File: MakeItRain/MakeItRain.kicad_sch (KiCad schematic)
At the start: 13 parts, among them IC1 DS3231SN#, J1 Conn_02x16_Odd_Even, J2 Conn_02x19_Odd_Even, J3 Conn_01x19, U2 S8411-45R

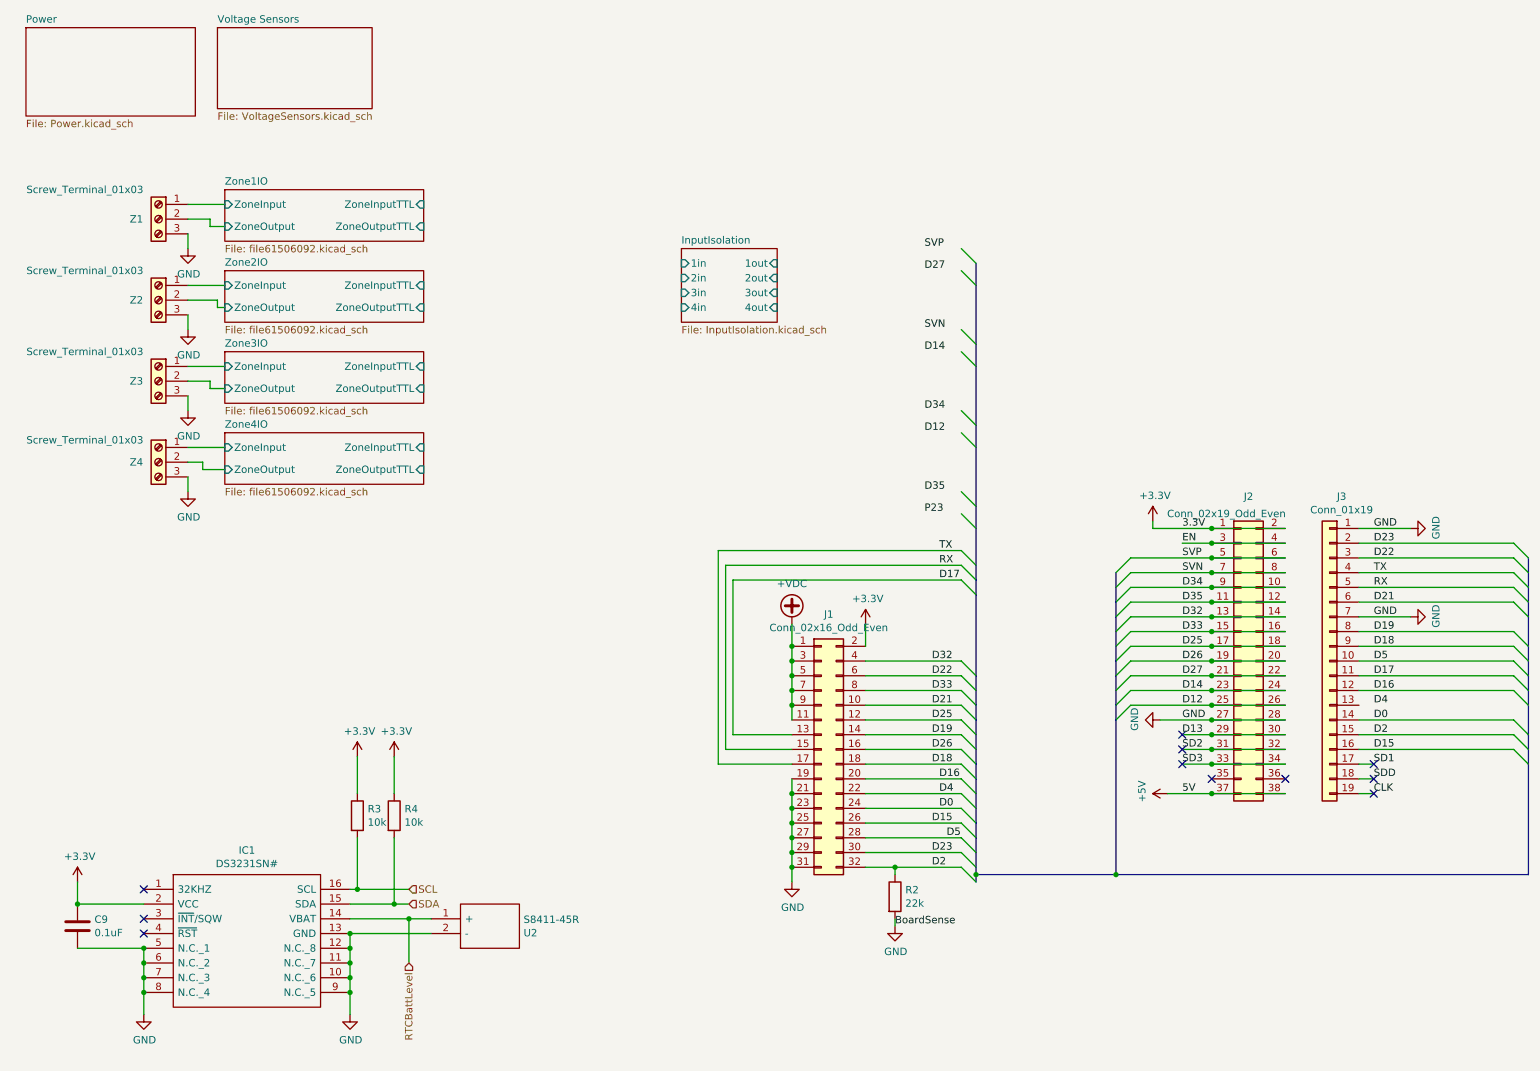
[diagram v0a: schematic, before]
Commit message: wip for input fix.
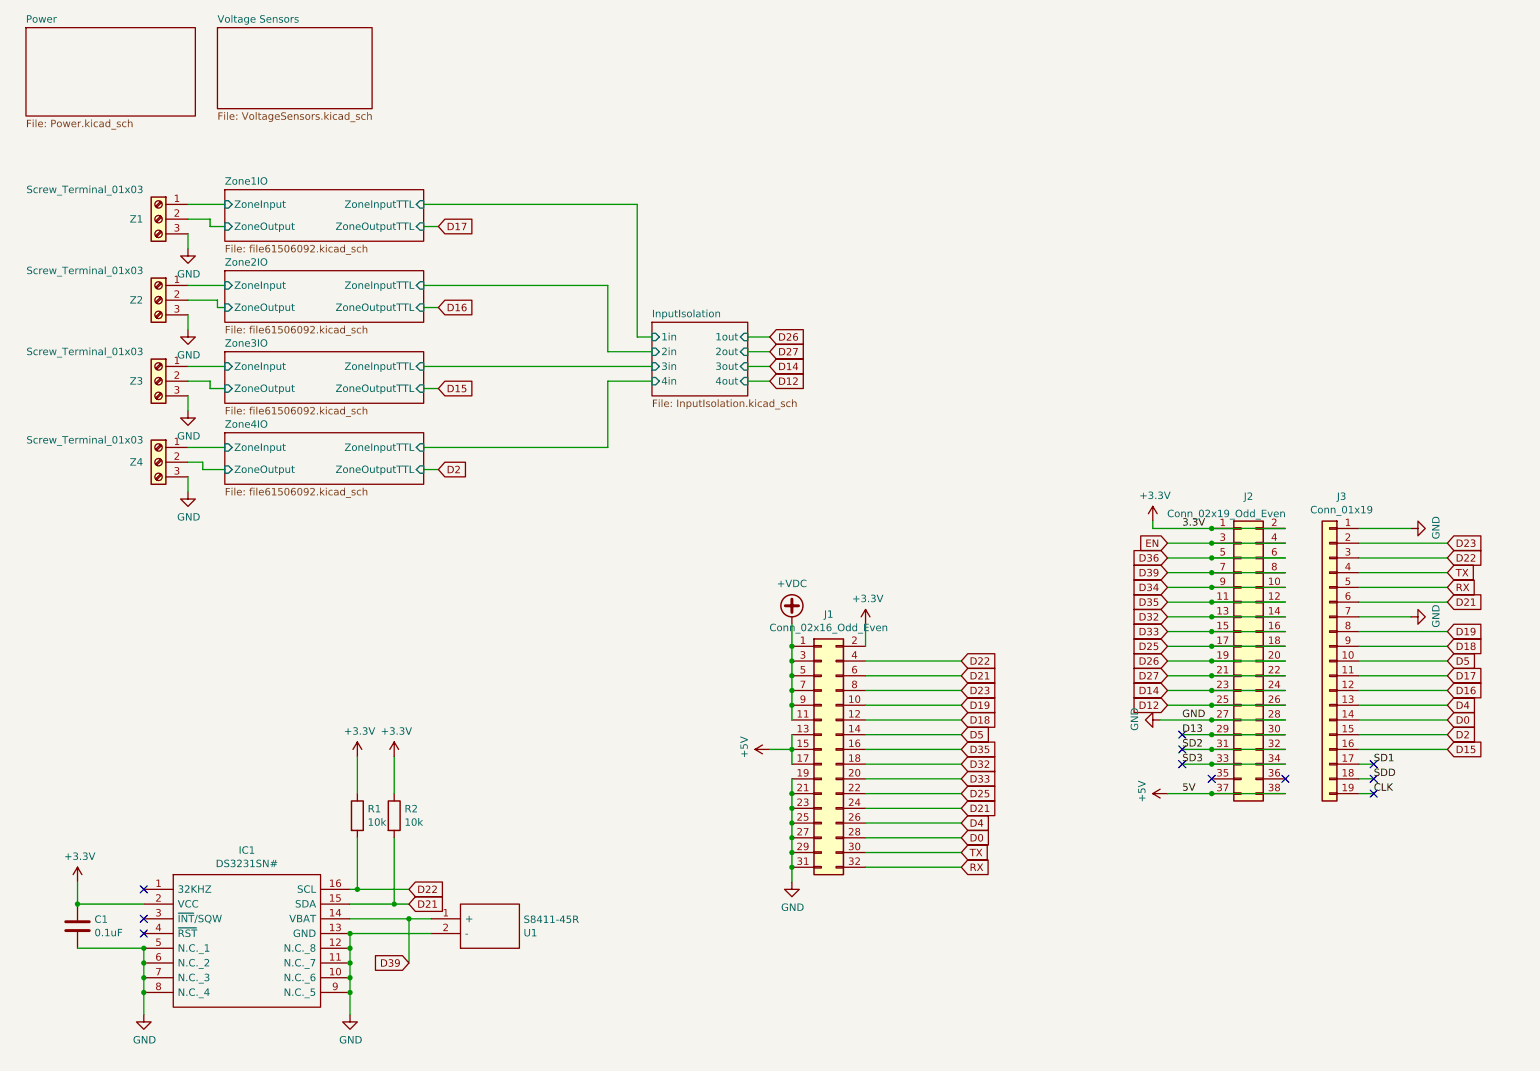
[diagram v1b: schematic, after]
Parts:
- removed R2: 22k, Resistor_THT:R_Axial_DIN0207_L6.3mm_D2.5mm_P5.08mm_Vertical, symbol Device:R
- renumbered C9 to C1, R3 to R1, R4 to R2, U2 to U1
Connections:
- net SCL is gone; now on net D22: IC1.16 (SCL), R1.2
- net SDA is gone; now on net D21: IC1.15 (SDA), R2.2
- net SVN is gone; now on net D39: J2.7 (Pin_7), J2.8 (Pin_8)
- net +5V: now also J1.13 (Pin_13), J1.15 (Pin_15), J1.17 (Pin_17)
- net D0: now also J1.28 (Pin_28); no longer J1.24 (Pin_24)
- net D15: no longer J1.26 (Pin_26)
- net D16: no longer J1.20 (Pin_20)
- net D17: no longer J1.13 (Pin_13)
- net D18: now also J1.12 (Pin_12); no longer J1.18 (Pin_18)
- net D19: now also J1.10 (Pin_10); no longer J1.14 (Pin_14)
- net D2: no longer J1.32 (Pin_32)
- net D21: now also J1.24 (Pin_24), J1.6 (Pin_6); no longer J1.10 (Pin_10)
- net D22: now also J1.4 (Pin_4); no longer J1.6 (Pin_6)
- net D23: now also J1.8 (Pin_8); no longer J1.30 (Pin_30)
- net D25: now also J1.22 (Pin_22); no longer J1.12 (Pin_12)
- net D26: no longer J1.16 (Pin_16)
- net D32: now also J1.18 (Pin_18); no longer J1.4 (Pin_4)
- net D33: now also J1.20 (Pin_20); no longer J1.8 (Pin_8)
- net D35: now also J1.16 (Pin_16)
- net D4: now also J1.26 (Pin_26), J3.13 (Pin_13); no longer J1.22 (Pin_22)
- net D5: now also J1.14 (Pin_14); no longer J1.28 (Pin_28)
- net RX: now also J1.32 (Pin_32); no longer J1.15 (Pin_15)
- net TX: now also J1.30 (Pin_30); no longer J1.17 (Pin_17)
- net RTCBattLevel renamed D39
- net SVP renamed D36

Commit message: wip for layout
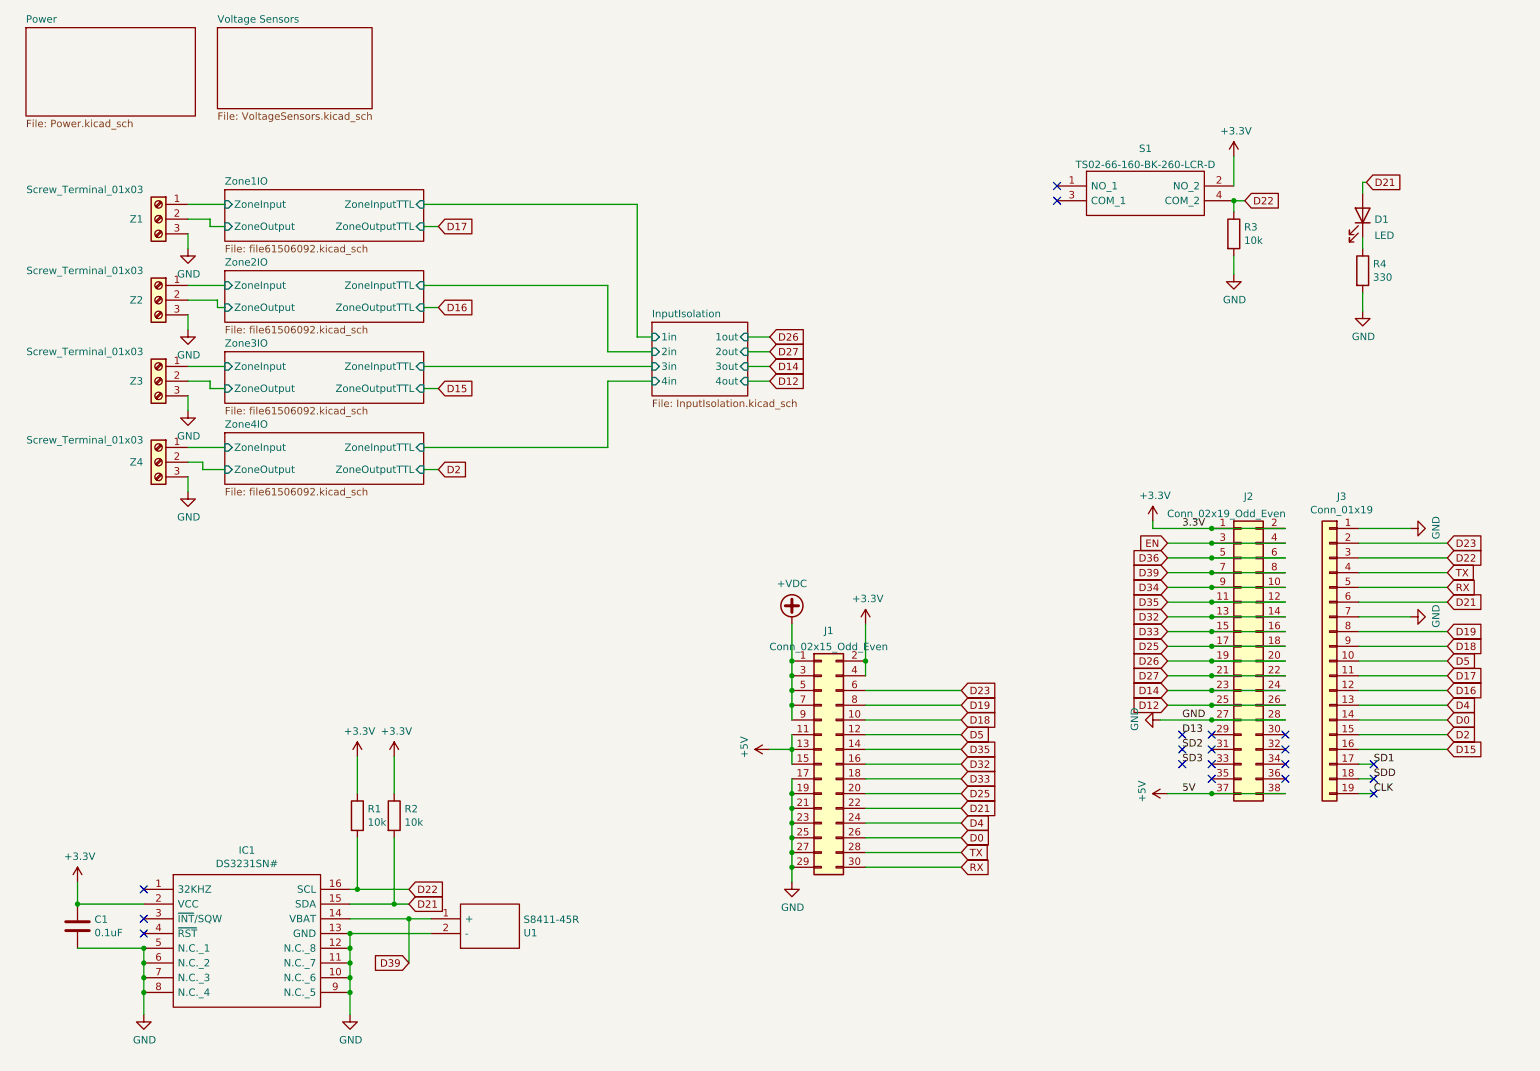
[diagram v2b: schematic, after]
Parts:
- removed J1: Conn_02x16_Odd_Even, Connector_PinSocket_2.54mm:PinSocket_2x16_P2.54mm_Vertical, symbol Connector_Generic:Conn_02x16_Odd_Even
- added D1: LED, LED_THT:LED_D3.0mm, symbol Device:LED
- added J1: Conn_02x15_Odd_Even, Connector_PinHeader_2.54mm:PinHeader_2x15_P2.54mm_Vertical, symbol Connector_Generic:Conn_02x15_Odd_Even
- added R3: 10k, Resistor_THT:R_Axial_DIN0207_L6.3mm_D2.5mm_P2.54mm_Vertical, symbol Device:R
- added R4: 330, Resistor_THT:R_Axial_DIN0207_L6.3mm_D2.5mm_P2.54mm_Vertical, symbol Device:R
- added S1: TS02-66-160-BK-260-LCR-D, TS0266160BK260LCRD, symbol Samac_Sys:TS02-66-160-BK-260-LCR-D
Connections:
- net +3V3: now also J1.2 (Pin_2), J1.4 (Pin_4), S1.2 (NO_2)
- net +5V: now also J1.11 (Pin_11), J1.13 (Pin_13), J1.15 (Pin_15)
- net +VDC: now also J1.1 (Pin_1), J1.3 (Pin_3), J1.5 (Pin_5), J1.7 (Pin_7), J1.9 (Pin_9)
- net D0: now also J1.26 (Pin_26)
- net D13: no longer J2.29 (Pin_29), J2.30 (Pin_30)
- net D18: now also J1.10 (Pin_10)
- net D19: now also J1.8 (Pin_8)
- net D21: now also D1.2 (A), J1.22 (Pin_22)
- net D22: now also R3.1, S1.4 (COM_2)
- net D23: now also J1.6 (Pin_6)
- net D25: now also J1.20 (Pin_20)
- net D32: now also J1.16 (Pin_16)
- net D33: now also J1.18 (Pin_18)
- net D35: now also J1.14 (Pin_14)
- net D4: now also J1.24 (Pin_24)
- net D5: now also J1.12 (Pin_12)
- net GND: now also J1.17 (Pin_17), J1.19 (Pin_19), J1.21 (Pin_21), J1.23 (Pin_23), J1.25 (Pin_25), J1.27 (Pin_27), J1.29 (Pin_29), R3.2, R4.2
- net RX: now also J1.30 (Pin_30)
- net SD2: no longer J2.31 (Pin_31), J2.32 (Pin_32)
- net SD3: no longer J2.33 (Pin_33), J2.34 (Pin_34)
- net TX: now also J1.28 (Pin_28)
- new net: D1.1 (K), R4.1
- no-connect marks 11 -> 19
